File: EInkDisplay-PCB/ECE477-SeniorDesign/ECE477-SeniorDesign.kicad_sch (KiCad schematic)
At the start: 0 parts

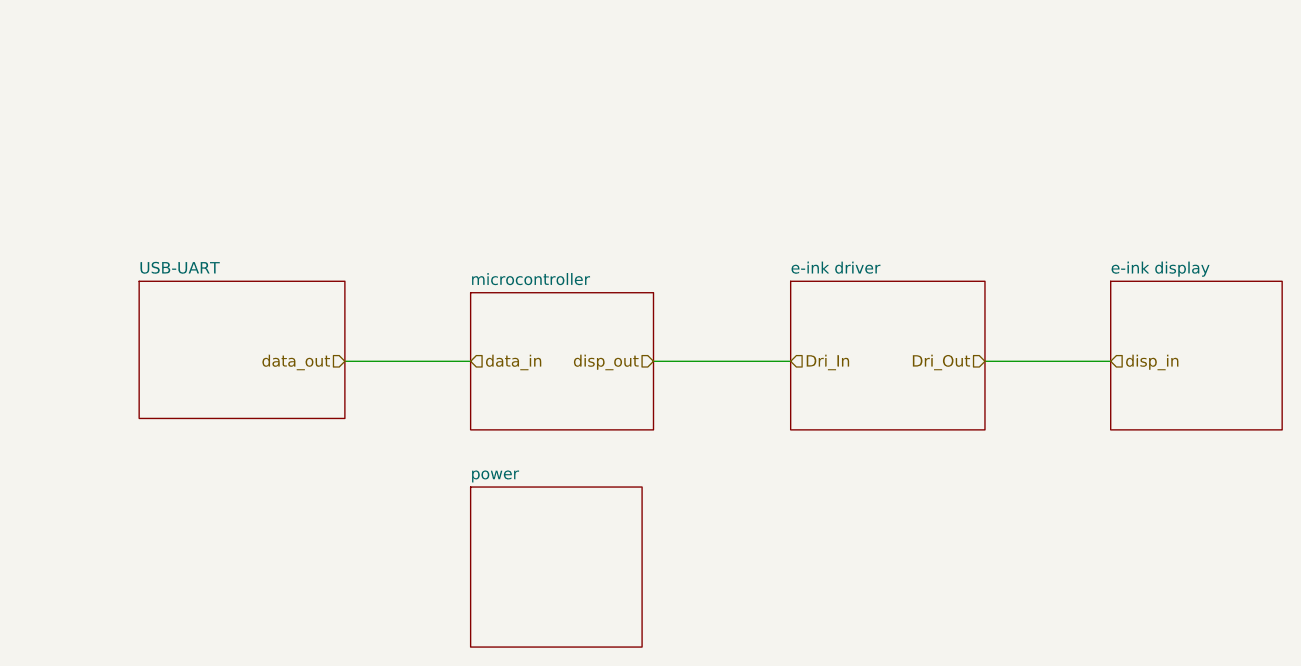
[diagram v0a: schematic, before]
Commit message: Update
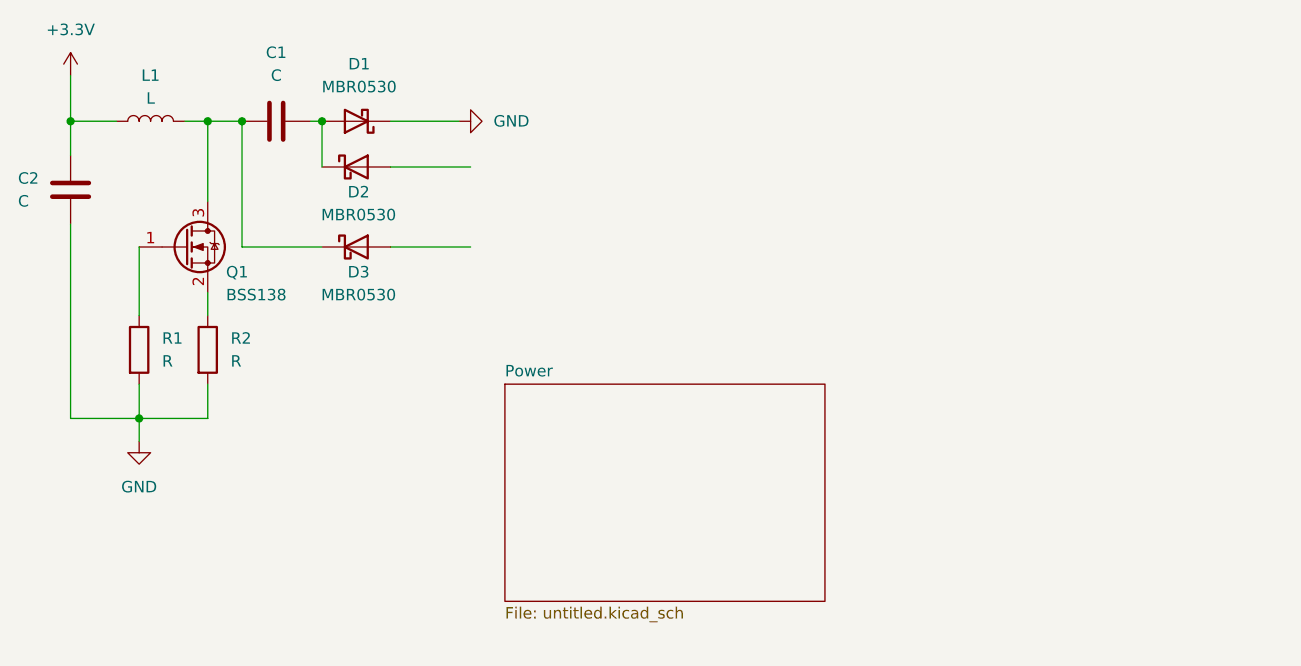
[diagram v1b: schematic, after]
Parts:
- added C1, C2: C, symbol Device:C
- added D1, D2, D3: MBR0530, Diode_SMD:D_SOD-123, symbol Diode:MBR0530
- added L1: L, symbol Device:L
- added Q1: BSS138, Package_TO_SOT_SMD:SOT-23, symbol Transistor_FET:BSS138
- added R1, R2: R, symbol Device:R
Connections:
- new net: C1.1, D3.1 (K), L1.2, Q1.3 (D)
- new net: C1.2, D1.2 (A), D2.1 (K)
- new net: Q1.1 (G), R1.1
- new net: Q1.2 (S), R2.1
- new net +3.3V: C2.1, L1.1
- new net GND: C2.2, D1.1 (K), R1.2, R2.2
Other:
- removed sheet USB-UART
- removed sheet e-ink display
- removed sheet e-ink driver
- removed sheet microcontroller
- removed sheet power
- added sheet Power (untitled.kicad_sch)
